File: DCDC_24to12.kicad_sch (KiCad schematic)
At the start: 26 parts, among them J1 Power_IN, J2 Power_OUT, U1 BD9F800MUX-ZE2

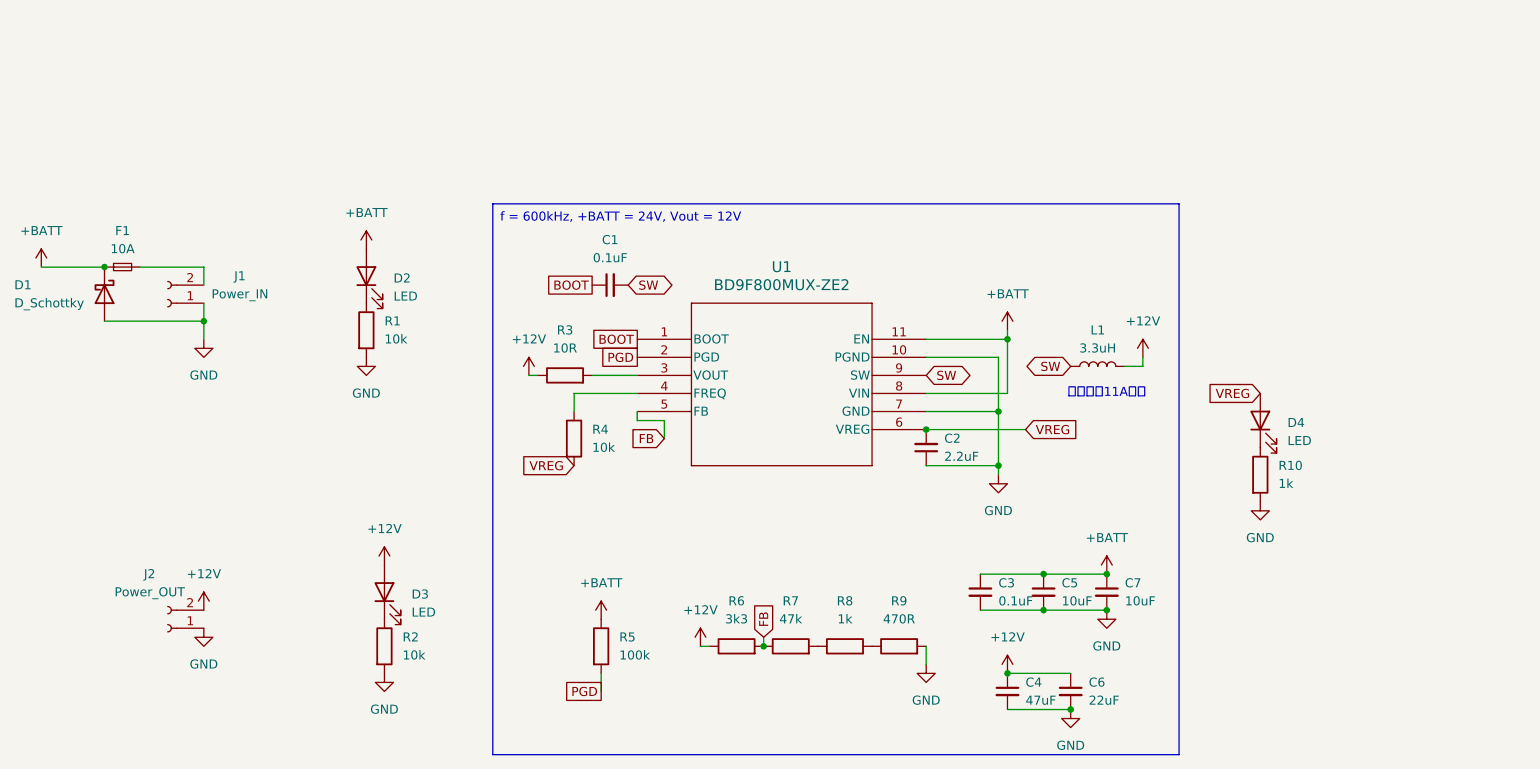
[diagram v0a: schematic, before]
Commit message: ノーテーション改善
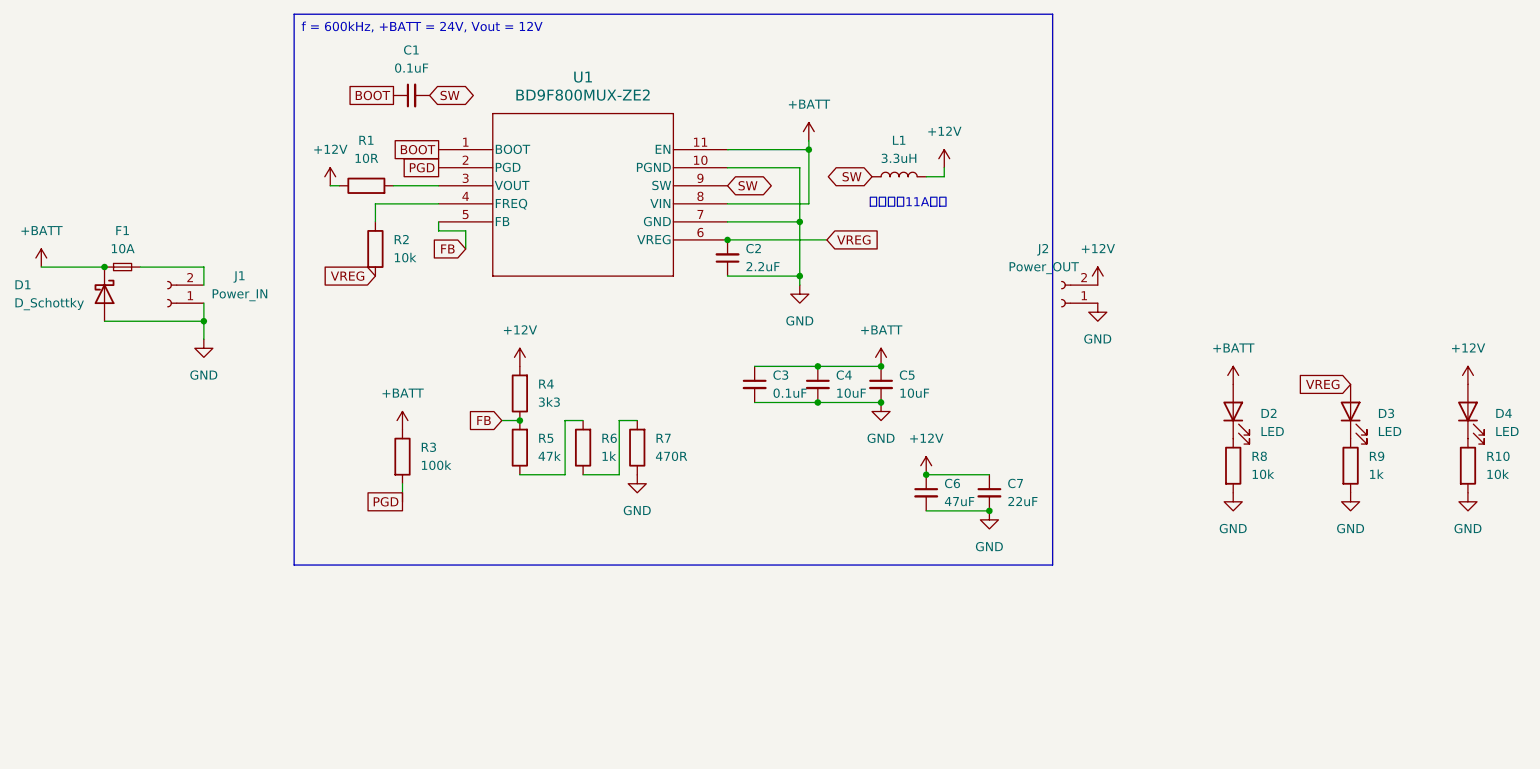
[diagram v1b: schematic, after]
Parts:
- renumbered C5 to C4, C7 to C5, C4 to C6, C6 to C7, D4 to D3, D3 to D4, R3 to R1, R2 to R10, R4 to R2, R5 to R3, R6 to R4, R7 to R5, R8 to R6, R9 to R7, R1 to R8, R10 to R9
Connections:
- net +12V: now also R4.2; no longer R4.1
- net FB: now also R4.1, R5.2; no longer R4.2, R5.1
- net GND: now also R7.1; no longer R7.2
- net at R6.1: now also R7.2; no longer R5.2
- net at R6.2: now also R5.1; no longer R7.1
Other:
- moved on the sheet: C1, C2, C3, C4, C5, C6, C7, D2, D3, D4, J2, L1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
